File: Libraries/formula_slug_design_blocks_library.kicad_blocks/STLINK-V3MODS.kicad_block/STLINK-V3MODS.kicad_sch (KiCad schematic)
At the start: 2 parts

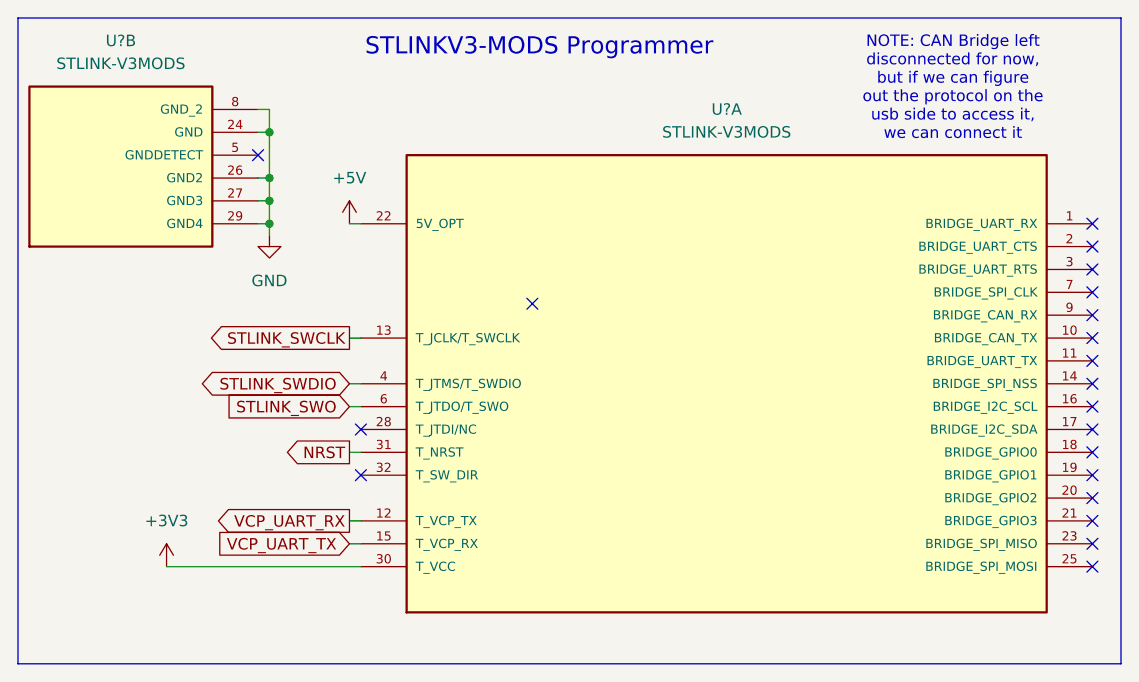
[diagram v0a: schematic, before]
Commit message: Fix symbol
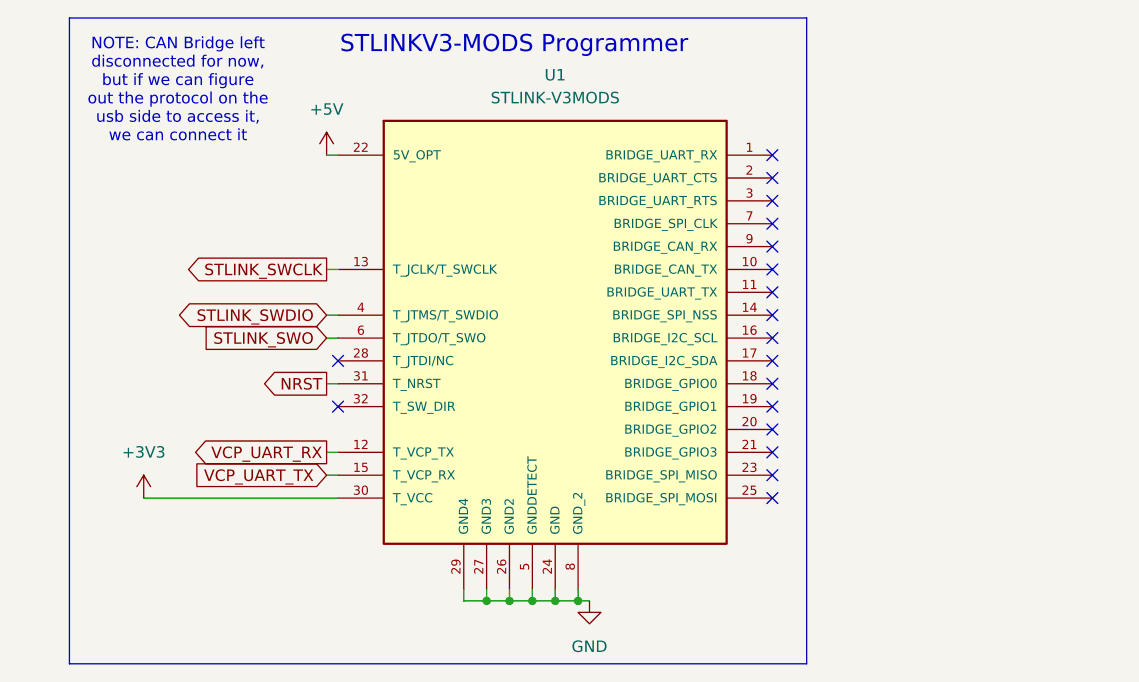
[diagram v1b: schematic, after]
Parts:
- removed U? (x2): STLINK-V3MODS, FS_4_Global_Footprint_Library:MODULE_STLINK-V3MODS, symbol FS_4_Global_Symbol_Library:STLINK-V3MODS
- added U1: STLINK-V3MODS, FS_4_Global_Footprint_Library:MODULE_STLINK-V3MODS, symbol FS_4_Global_Symbol_Library:STLINK-V3MODS
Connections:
- net +3V3: now also U1.30 (T_VCC)
- net +5V: now also U1.22 (5V_OPT)
- net GND: now also U1.24 (GND), U1.26 (GND2), U1.27 (GND3), U1.29 (GND4), U1.5 (GNDDETECT), U1.8 (GND_2)
- net NRST: now also U1.31 (T_NRST)
- net STLINK_SWCLK: now also U1.13 (T_JCLK/T_SWCLK)
- net STLINK_SWDIO: now also U1.4 (T_JTMS/T_SWDIO)
- net STLINK_SWO: now also U1.6 (T_JTDO/T_SWO)
- net VCP_UART_RX: now also U1.12 (T_VCP_TX)
- net VCP_UART_TX: now also U1.15 (T_VCP_RX)
- no-connect marks 20 -> 18
